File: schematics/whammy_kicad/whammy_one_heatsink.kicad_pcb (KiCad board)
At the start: 2 copper layers, 49 parts, among them Q1 2SK2013, Q2 2SJ313, Q3 2SK2013, Q4 2SJ313, U1 OPA2604, U4 4N35, U5 4N35

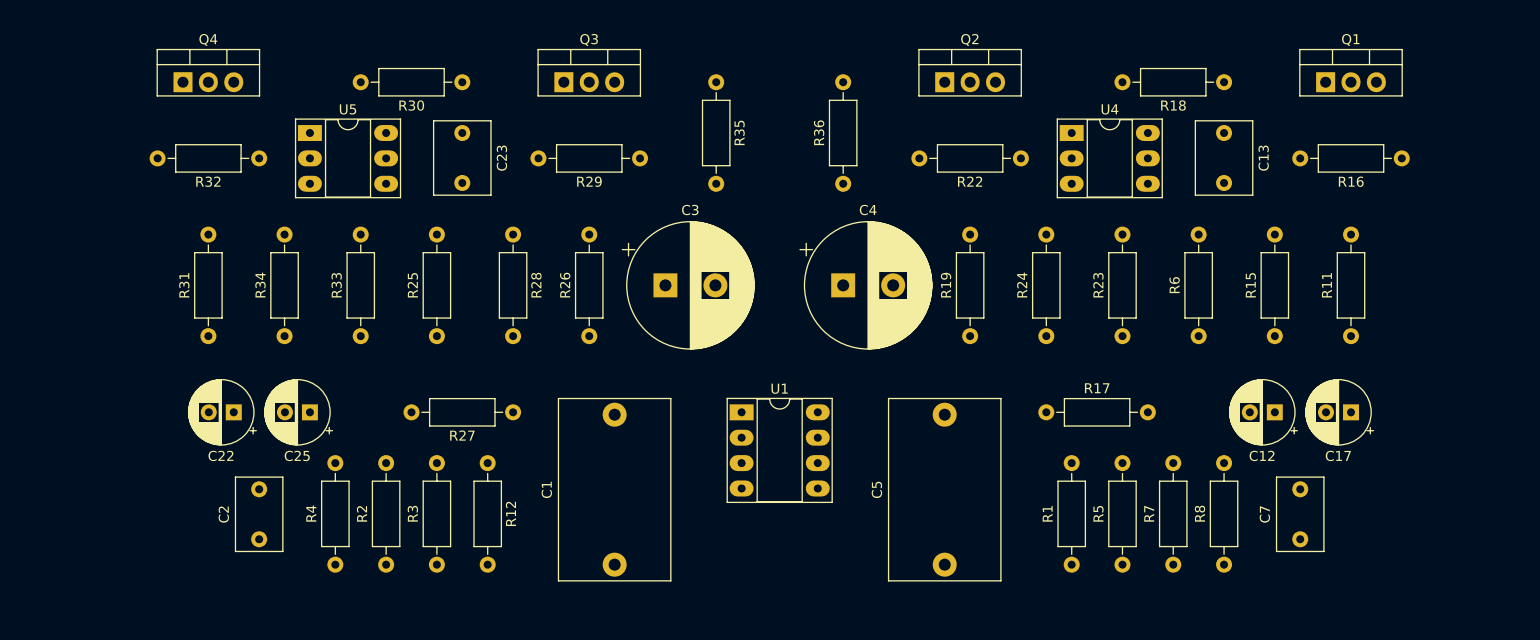
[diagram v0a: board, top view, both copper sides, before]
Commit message: Final version
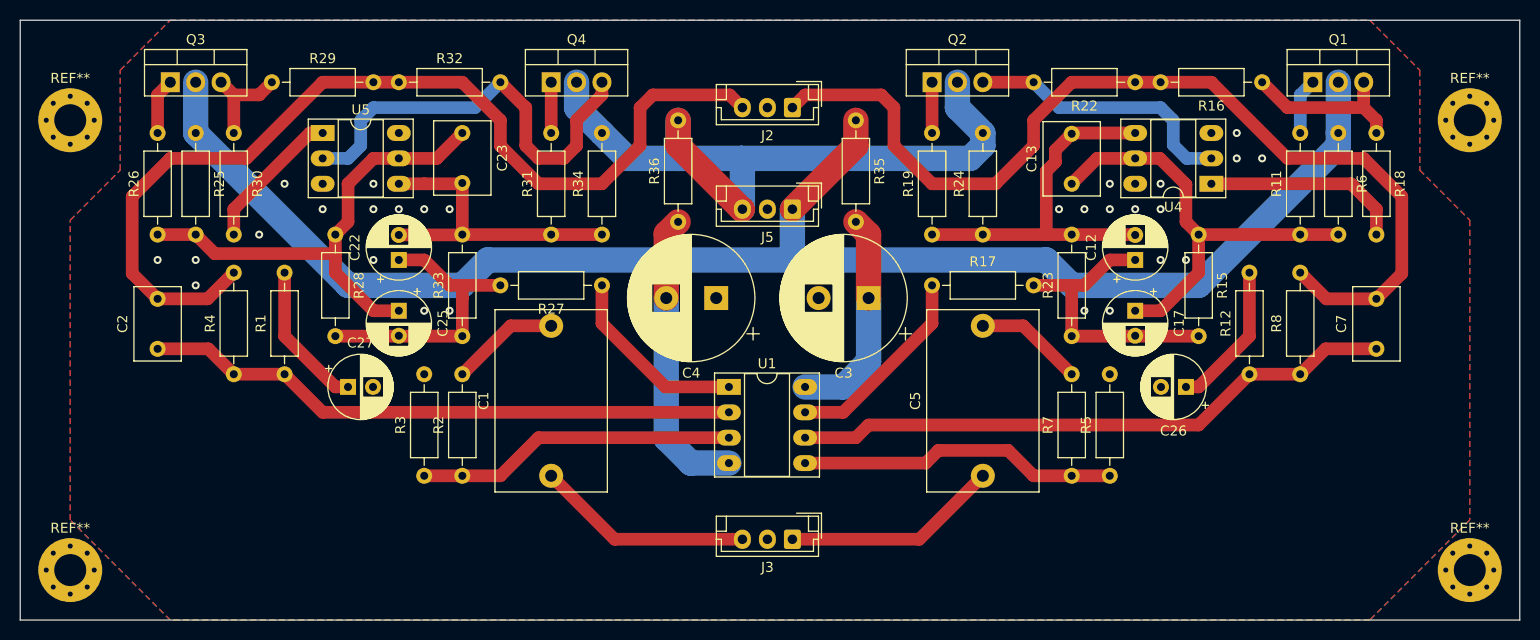
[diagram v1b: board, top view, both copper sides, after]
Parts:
- added C26: 22uF/25V, Capacitor_THT:CP_Radial_D6.3mm_P2.50mm, F.Cu at (181.6, 106.7)
- added C27: 22uF/25V, Capacitor_THT:CP_Radial_D6.3mm_P2.50mm, F.Cu at (97.8, 106.7)
- added J2: Conn_01x03, Connector_JST:JST_EH_B3B-EH-A_1x03_P2.50mm_Vertical, F.Cu at (142.2, 78.7)
- added J3: Conn_01x03, Connector_JST:JST_EH_B3B-EH-A_1x03_P2.50mm_Vertical, F.Cu at (142.2, 121.9)
- added J5: Conn_01x03, Connector_JST:JST_EH_B3B-EH-A_1x03_P2.50mm_Vertical, F.Cu at (142.2, 88.9)
- added REF**: MountingHole_3.2mm_M3_Pad_Via, MountingHole:MountingHole_3.2mm_M3_Pad_Via, F.Cu at (70.0, 125.0)
- added REF**: MountingHole_3.2mm_M3_Pad_Via, MountingHole:MountingHole_3.2mm_M3_Pad_Via, F.Cu at (210.0, 125.0)
- added REF**: MountingHole_3.2mm_M3_Pad_Via, MountingHole:MountingHole_3.2mm_M3_Pad_Via, F.Cu at (210.0, 80.0)
- added REF**: MountingHole_3.2mm_M3_Pad_Via, MountingHole:MountingHole_3.2mm_M3_Pad_Via, F.Cu at (70.0, 80.0)
- moved R1 81.0 mm to (91.4, 105.4)
- moved R12 76.7 mm to (188.0, 105.4), turned to 90 degrees
- moved R26 44.4 mm to (78.7, 91.4)
- moved Q3 39.4 mm to (80.0, 76.2)
- moved R29 37.6 mm to (90.2, 76.2), turned to 0 degrees
- moved Q4 36.8 mm to (118.1, 76.2)
- moved R31 35.8 mm to (118.1, 91.4)
- moved R34 33.3 mm to (123.2, 91.4)
- moved R25 31.5 mm to (82.5, 81.3), turned to 270 degrees
- moved R6 24.7 mm to (196.8, 81.3), turned to 270 degrees
- moved C17 23.9 mm to (176.5, 99.1), turned to 270 degrees
- moved R30 23.4 mm to (86.4, 81.3), turned to 270 degrees
- moved C22 22.5 mm to (102.9, 94.0), turned to 90 degrees
- moved C2 21.6 mm to (78.7, 102.9)
- moved R4 21.6 mm to (86.4, 105.4)
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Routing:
- net +15V: track 0.00 -> 156.5 mm
- net RIGHT_OUT: track 0.00 -> 97.9 mm
- net LEFT_OUT: track 0.00 -> 97.8 mm
- net -15V: track 0.00 -> 73.7 mm
- net Net-(C7-Pad1): track 0.00 -> 60.8 mm
- net Net-(C2-Pad1): track 0.00 -> 59.8 mm
- net Net-(C23-Pad1): track 0.00 -> 49.8 mm
- net Net-(C13-Pad1): track 0.00 -> 44.8 mm
- net Net-(Q4-Pad3): track 0.00 -> 43.4 mm
- net Net-(C12-Pad2): track 0.00 -> 37.9 mm
- net Net-(R5-Pad1): track 0.00 -> 32.1 mm
- net Net-(R2-Pad1): track 0.00 -> 32.1 mm
- net Net-(C22-Pad2): track 0.00 -> 31.9 mm
- net Net-(C4-Pad2): track 0.00 -> 29.5 mm
- net Net-(C22-Pad1): track 0.00 -> 29.0 mm
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- added copper zone on B.Cu, net GND
- added copper zone on F.Cu, net GND
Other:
- board outline added: 150 x 60 mm
